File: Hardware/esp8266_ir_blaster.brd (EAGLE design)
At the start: 25.4 x 27.6 mm, 43 parts, among them Q1 600mA/40V, U1 ESP-12S, U2 38kHz

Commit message: Revising LED color. Adding production panel.
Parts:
- D2: value BLUE -> GREEN
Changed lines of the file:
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@@
 <?xml version="1.0" encoding="utf-8"?>
 <!DOCTYPE eagle SYSTEM "eagle.dtd">
-<eagle version="9.0.1">
+<eagle version="9.1.1">
 <drawing>
 <settings>
@@
 <layer number="23" name="tOrigins" color="15" fill="1" visible="yes" active="yes"/>
 <layer number="24" name="bOrigins" color="15" fill="1" visible="yes" active="yes"/>
-<layer number="25" name="tNames" color="7" fill="1" visible="no" active="yes"/>
-<layer number="26" name="bNames" color="7" fill="1" visible="no" active="yes"/>
-<layer number="27" name="tValues" color="7" fill="1" visible="no" active="yes"/>
-<layer number="28" name="bValues" color="7" fill="1" visible="no" active="yes"/>
-<layer number="29" name="tStop" color="7" fill="3" visible="no" active="yes"/>
-<layer number="30" name="bStop" color="7" fill="6" visible="no" active="yes"/>
-<layer number="31" name="tCream" color="7" fill="4" visible="no" active="yes"/>
-<layer number="32" name="bCream" color="7" fill="5" visible="no" active="yes"/>
-<layer number="33" name="tFinish" color="6" fill="3" visible="no" active="yes"/>
-<layer number="34" name="bFinish" color="6" fill="6" visible="no" active="yes"/>
-<layer number="35" name="tGlue" color="7" fill="4" visible="no" active="yes"/>
-<layer number="36" name="bGlue" color="7" fill="5" visible="no" active="yes"/>
-<layer number="37" name="tTest" color="7" fill="1" visible="no" active="yes"/>
-<layer number="38" name="bTest" color="7" fill="1" visible="no" active="yes"/>
+<layer number="25" name="tNames" color="7" fill="1" visible="yes" active="yes"/>
+<layer number="26" name="bNames" color="7" fill="1" visible="yes" active="yes"/>
+<layer number="27" name="tValues" color="7" fill="1" visible="yes" active="yes"/>
+<layer number="28" name="bValues" color="7" fill="1" visible="yes" active="yes"/>
+<layer number="29" name="tStop" color="7" fill="3" visible="yes" active="yes"/>
+<layer number="30" name="bStop" color="7" fill="6" visible="yes" active="yes"/>
+<layer number="31" name="tCream" color="7" fill="4" visible="yes" active="yes"/>
+<layer number="32" name="bCream" color="7" fill="5" visible="yes" active="yes"/>
+<layer number="33" name="tFinish" color="6" fill="3" visible="yes" active="yes"/>
+<layer number="34" name="bFinish" color="6" fill="6" visible="yes" active="yes"/>
+<layer number="35" name="tGlue" color="7" fill="4" visible="yes" active="yes"/>
+<layer number="36" name="bGlue" color="7" fill="5" visible="yes" active="yes"/>
+<layer number="37" name="tTest" color="7" fill="1" visible="yes" active="yes"/>
+<layer number="38" name="bTest" color="7" fill="1" visible="yes" active="yes"/>
 <layer number="39" name="tKeepout" color="4" fill="11" visible="yes" active="yes"/>
-<layer number="40" name="bKeepout" color="1" fill="11" visible="no" active="yes"/>
-<layer number="41" name="tRestrict" color="4" fill="10" visible="no" active="yes"/>
-<layer number="42" name="bRestrict" color="1" fill="10" visible="no" active="yes"/>
-<layer number="43" name="vRestrict" color="2" fill="10" visible="no" active="yes"/>
-<layer number="44" name="Drills" color="7" fill="1" visible="no" active="yes"/>
-<layer number="45" name="Holes" color="7" fill="1" visible="no" active="yes"/>
-<layer number="46" name="Milling" color="3" fill="1" visible="no" active="yes"/>
-<layer number="47" name="Measures" color="7" fill="1" visible="no" active="yes"/>
-<layer number="48" name="Document" color="7" fill="1" visible="no" active="yes"/>
-<layer number="49" name="Reference" color="7" fill="1" visible="no" active="yes"/>
-<layer number="50" name="dxf" color="7" fill="1" visible="no" active="yes"/>
+<layer number="40" name="bKeepout" color="1" fill="11" visible="yes" active="yes"/>
+<layer number="41" name="tRestrict" color="4" fill="10" visible="yes" active="yes"/>
+<layer number="42" name="bRestrict" color="1" fill="10" visible="yes" active="yes"/>
+<layer number="43" name="vRestrict" color="2" fill="10" visible="yes" active="yes"/>
+<layer number="44" name="Drills" color="7" fill="1" visible="yes" active="yes"/>
+<layer number="45" name="Holes" color="7" fill="1" visible="yes" active="yes"/>
+<layer number="46" name="Milling" color="3" fill="1" visible="yes" active="yes"/>
+<layer number="47" name="Measures" color="7" fill="1" visible="yes" active="yes"/>
+<layer number="48" name="Document" color="7" fill="1" visible="yes" active="yes"/>
+<layer number="49" name="Reference" color="7" fill="1" visible="yes" active="yes"/>
+<layer number="50" name="dxf" color="7" fill="1" visible="yes" active="yes"/>
 <layer number="51" name="tDocu" color="6" fill="1" visible="yes" active="yes"/>
-<layer number="52" name="bDocu" color="7" fill="1" visible="no" active="yes"/>
+<layer number="52" name="bDocu" color="7" fill="1" visible="yes" active="yes"/>
 <layer number="91" name="Nets" color="2" fill="1" visible="no" active="no"/>
 <layer number="92" name="Busses" color="1" fill="1" visible="no" active="no"/>
@@
 <param name="checkStop" value="0"/>
 <param name="checkValues" value="0"/>
+<param name="checkNames" value="1"/>
+<param name="checkWireStubs" value="1"/>
+<param name="checkPolygonWidth" value="0"/>
 <param name="useDiameter" value="13"/>
 <param name="maxErrors" value="50"/>
@@
 <attribute name="PROD_ID" value="RES-07856" x="14.351" y="15.875" size="1.778" layer="27" font="vector" ratio="15" rot="R90" display="off"/>
 </element>
-<element name="D2" library="SparkFun-LED" package="LED-0603" value="BLUE" x="12.7" y="15.875" rot="R90">
-<attribute name="PROD_ID" value="DIO-08575" x="12.7" y="15.875" size="1.778" layer="27" font="vector" ratio="15" rot="R90" display="off"/>
+<element name="D2" library="SparkFun-LED" package="LED-0603" value="GREEN" x="12.7" y="15.875" rot="R90">
+<attribute name="PROD_ID" value="DIO-00821" x="12.7" y="15.875" size="1.778" layer="27" font="vector" ratio="15" rot="R90" display="off"/>
 </element>
 <element name="Q1" library="SparkFun-DiscreteSemi" package="SOT23-3" value="600mA/40V" x="13.97" y="5.08" rot="R90">
@@
 </signal>
 </signals>
+<mfgpreviewcolors>
+<mfgpreviewcolor name="soldermaskcolor" color="0xC8008000"/>
+<mfgpreviewcolor name="silkscreencolor" color="0xFFFEFEFE"/>
+<mfgpreviewcolor name="backgroundcolor" color="0xFF282828"/>
+<mfgpreviewcolor name="coppercolor" color="0xFFFFBF00"/>
+<mfgpreviewcolor name="substratecolor" color="0xFF786E46"/>
+</mfgpreviewcolors>
 </board>
 </drawing>

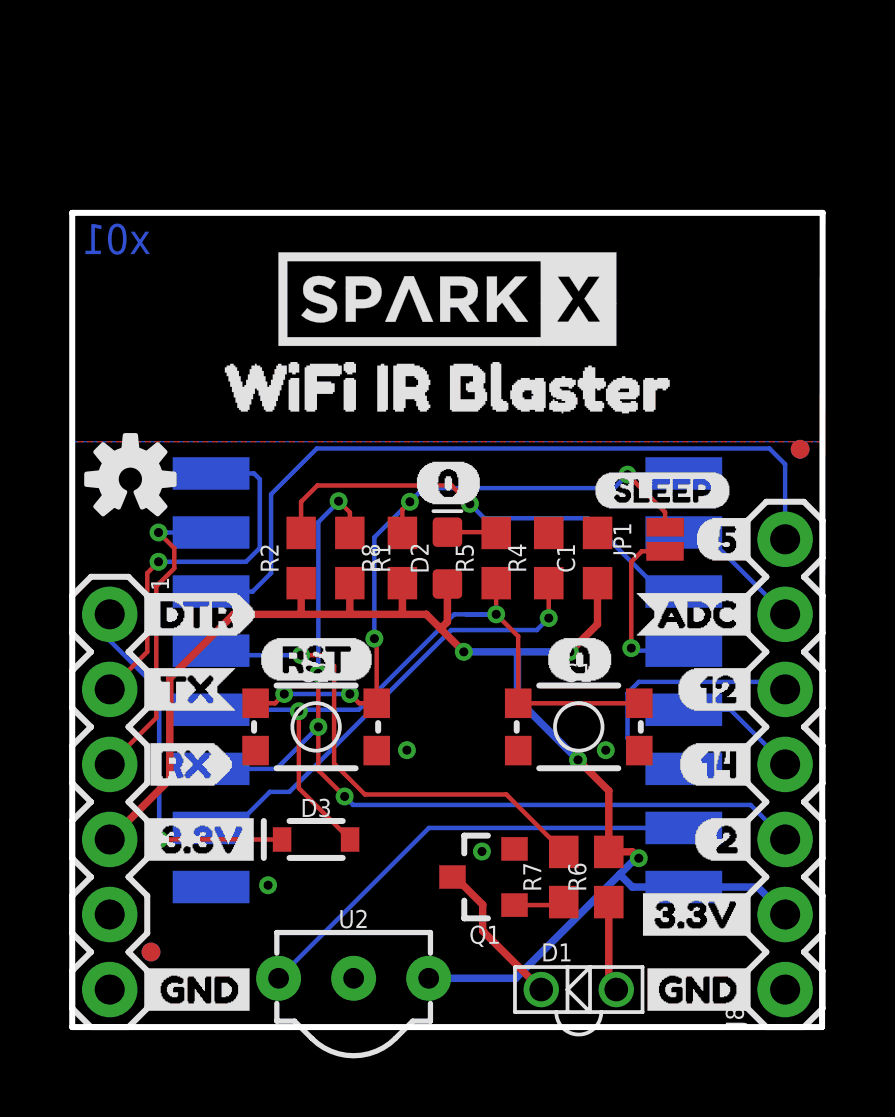
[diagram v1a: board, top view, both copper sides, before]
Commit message: x02 hardware commit
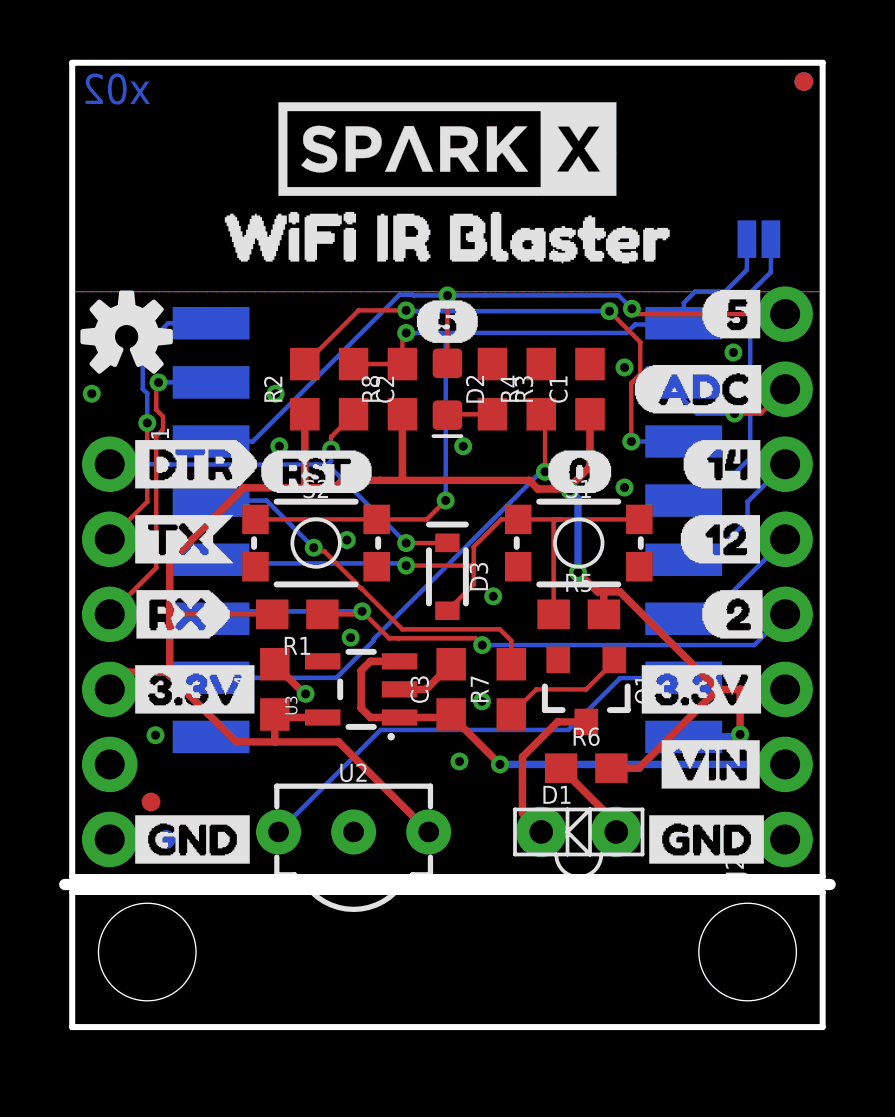
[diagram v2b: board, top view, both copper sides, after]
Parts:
- removed J8: (no value), SparkFun-Connectors:1X07
- removed U$16: (no value), buzzard_labels:013
- removed U$17: (no value), buzzard_labels:SLEEP15
- removed U$7: (no value), buzzard_labels:58
- added C2, C3: 1.0uF, SparkFun-Capacitors:0603
- added C4: 2.2uF, SparkFun-Capacitors:0603
- added H1, H2: STAND-OFF, SparkFun-Hardware:STAND-OFF
- added J2: (no value), SparkFun-Connectors:1X08_NO_SILK
- added R3: 1k, SparkFun-Resistors:0603
- added U$19: (no value), buzzard_labels:TX2
- added U$20: (no value), buzzard_labels:RX3
- added U$21: (no value), buzzard_labels:3#3V4
- added U$22, U$24: (no value), buzzard_labels:GND5
- added U$23: (no value), buzzard_labels:VIN6
- added U3: 3.3V, SparkFun-IC-Power:SOT23-5
- J1: device SparkFun-Connectors:1X06 -> SparkFun-Connectors:1X06_NO_SILK
- R6: value 68 -> 20
- U$1: device buzzard_labels:GND11 -> buzzard_labels:512
- U$10: device buzzard_labels:RX3 -> buzzard_labels:129
- U$11: device buzzard_labels:TX4 -> buzzard_labels:148
- U$12: device buzzard_labels:DTR5 -> buzzard_labels:27
- U$2: device buzzard_labels:3#3V12 -> buzzard_labels:3#3V4
- U$3: device buzzard_labels:210 -> buzzard_labels:SLP14
- U$4: device buzzard_labels:149 -> buzzard_labels:WIFI_IR_BLASTER11
- U$5: device buzzard_labels:127 -> buzzard_labels-02:UART0
- U$6: device buzzard_labels:ADC6 -> buzzard_labels:DTR1
- U$8: device buzzard_labels:GND1 -> buzzard_labels:511
- U$9: device buzzard_labels:3#3V2 -> buzzard_labels:ADC10
- moved U$8 29.7 mm to (21.2, 24.1)
- moved U$1 23.8 mm to (11.6, 23.9)
- moved U$9 22.6 mm to (18.9, 21.6)
- moved U$3 22.2 mm to (25.1, 28.2), flipped to the bottom
- moved U$5 21.4 mm to (1.27, 20.8), flipped to the bottom, turned to 90 degrees
- moved U$11 19.9 mm to (20.6, 19.1)
- moved U$10 19.7 mm to (20.3, 16.5)
- moved U$12 19.2 mm to (21.2, 14.0)
- moved U$6 18.1 mm to (1.65, 19.1)
- moved FD1 12.4 mm to (24.8, 32.0)
- moved FD4 12.4 mm to (24.8, 32.0)
- moved JP1 10.6 mm to (23.2, 26.7), flipped to the bottom, turned to 0 degrees
- moved D3 9.94 mm to (12.7, 15.2), turned to 270 degrees
- moved U$2 7.62 mm to (18.8, 11.4)
- moved Q1 7.22 mm to (17.4, 11.4), turned to 180 degrees
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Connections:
- removed net N$2: D2.C, R5.2
- new net N$1: D2.C, R3.2
- new net VIN: C3.1, J2.2, U3.1, U3.3
- net 3.3V: now also C4.1, J2.3, R5.2, U3.5; no longer D2.A, J8.2
- net ADC: now also J2.7; no longer J8.6
- net DTR: now also C2.2
- net GND: now also C3.2, C4.2, J2.1, R3.1, U3.2; no longer J8.1
- net IO12: now also J2.5; no longer J8.5
- net IO14: now also J2.6; no longer J8.4
- net IO2: now also J2.4; no longer J8.3
- net IO5: now also D2.A, J2.8; no longer J8.7
- net RESET: now also C2.1
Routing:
- net VIN: track 0.00 -> 17.9 mm, vias 0 -> 1
- net 3.3V: track 52.9 -> 67.1 mm, vias 4 -> 3
- net IO2: track 31.6 -> 21.8 mm, vias 4 -> 2
- net IO12: track 9.46 -> 4.54 mm
- net IO0: track 25.6 -> 20.9 mm, vias 2 -> 1
- net RESET: track 24.9 -> 29.1 mm, vias 5 -> 2
- net IR_OUT: track 16.7 -> 12.9 mm
- net IO16: track 6.83 -> 10.5 mm, vias 1 -> 0
- net GND: track 0.00 -> 3.56 mm, vias 4 -> 14
- net TXO: track 12.7 -> 9.71 mm
- net N$7: track 1.71 -> 4.29 mm
- net IO5: track 26.6 -> 24.1 mm, vias 0 -> 2
- net DTR: track 12.5 -> 14.6 mm, vias 1 -> 2
- net CHIP_EN: track 15.7 -> 17.8 mm, vias 1 -> 3
- net N$2: track 1.66 -> 0.00 mm
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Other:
- board size 25.4 x 27.6 mm -> 25.9 x 32.6 mm
- board text added: "x02"
- board text removed: "x01"
